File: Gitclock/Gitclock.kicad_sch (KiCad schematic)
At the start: 40 parts, among them J1 PJ-102AH, J2 Conn_01x06, J3 Conn_01x05, SW1 Omron_B3F_SPST, SW2 Omron_B3F_SPST, SW3 Omron_B3F_SPST, U1 ATmega328-PU, U2 L7805, U3 MAX7219, U4 DS1307_DIP-8, U5 WH2004A-CFH-JT#, Y1 Crystal_16MHz, Y2 Crystal_32768Hz

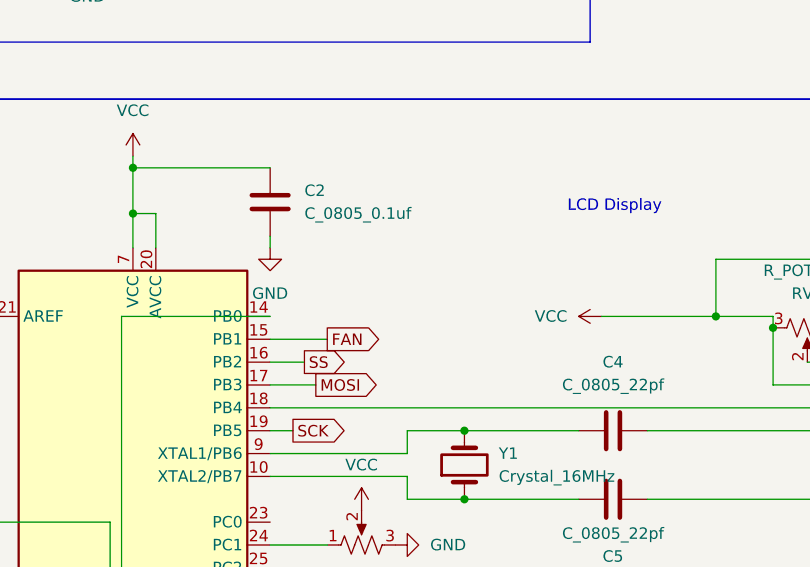
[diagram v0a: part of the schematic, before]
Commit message: gitclock
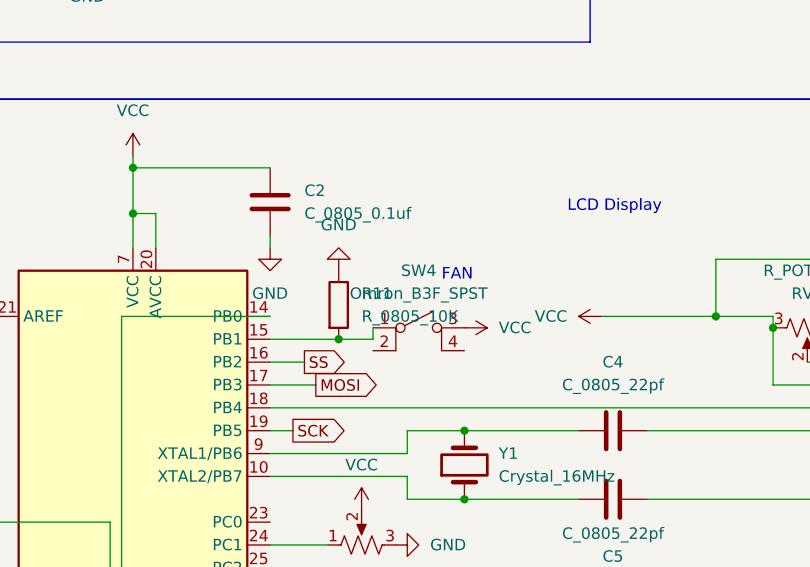
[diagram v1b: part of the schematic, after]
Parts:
- added R11: R_0805_10K, footprints:R_0805_2012Metric, symbol HPS:R_0805_10K
- added SW4: Omron_B3F_SPST, footprints:SW_SPST_Omron_B3FS-100xP, symbol HPS:Omron_B3F_SPST
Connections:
- net FAN: no longer U1.15 (PB1)
- net GND: now also R11.1
- net VCC: now also SW4.3 (B)
- new net: R11.2, SW4.1 (A), U1.15 (PB1)
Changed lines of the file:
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@@
   (junction (at 256.54 116.84) (diameter 0) (color 0 0 0 0)
+  )
+  (junction (at 203.2 99.06) (diameter 0) (color 0 0 0 0)
   )
   (no_connect (at 210.82 31.75))
@@
     (stroke (width 0) (type default) (color 0 0 0 0))
   )
+  (wire (pts (xy 207.01 99.06) (xy 207.01 97.79))
+    (stroke (width 0) (type default) (color 0 0 0 0))
+  )
   (wire (pts (xy 25.4 160.02) (xy 29.21 160.02))
     (stroke (width 0) (type default) (color 0 0 0 0))
@@
     (stroke (width 0) (type default) (color 0 0 0 0))
   )
+  (wire (pts (xy 203.2 99.06) (xy 207.01 99.06))
+    (stroke (width 0) (type default) (color 0 0 0 0))
+  )
   (wire (pts (xy 266.7 114.3) (xy 269.24 114.3))
     (stroke (width 0) (type default) (color 0 0 0 0))
@@
     (stroke (width 0) (type default) (color 0 0 0 0))
   )
-  (wire (pts (xy 195.58 99.06) (xy 201.93 99.06))
+  (wire (pts (xy 195.58 99.06) (xy 203.2 99.06))
     (stroke (width 0) (type default) (color 0 0 0 0))
   )
@@
   (text "MCU" (at 144.78 78.74 0)
     (effects (font (size 3 3)) (justify left bottom))
+  )
+  (text "FAN" (at 214.63 92.71 0)
+    (effects (font (size 1.27 1.27)) (justify left bottom))
   )
   (text "RTS\n" (at 237.49 20.32 0)
@@
     (effects (font (size 1.27 1.27)) (justify left))
     (property "Intersheet References" "${INTERSHEET_REFS}" (id 0) (at 169.4483 39.2906 0)
-      (effects (font (size 1.27 1.27)) (justify left) hide)
-    )
-  )
-  (global_label "FAN" (shape output) (at 201.93 99.06 0) (fields_autoplaced)
-    (effects (font (size 1.27 1.27)) (justify left))
-    (property "Intersheet References" "${INTERSHEET_REFS}" (id 0) (at 207.8507 98.9806 0)
       (effects (font (size 1.27 1.27)) (justify left) hide)
     )
@@
     )
     (property "Tolerance" "N/A" (id 10) (at 207.01 39.37 0)
+      (effects (font (size 1.27 1.27)) hide)
+    )
+    (pin "1")
+    (pin "2")
+  )
+  (symbol (lib_id "HPS:R_0805_10K") (at 203.2 95.25 0) (unit 1)
+    (in_bom yes) (on_board yes) (fields_autoplaced)
+    (property "Reference" "R11" (id 0) (at 205.74 93.9799 0)
+      (effects (font (size 1.27 1.27)) (justify left))
+    )
+    (property "Value" "R_0805_10K" (id 1) (at 205.74 96.5199 0)
+      (effects (font (size 1.27 1.27)) (justify left))
+    )
+    (property "Footprint" "footprints:R_0805_2012Metric" (id 2) (at 203.2 111.76 0)
+      (effects (font (size 1.27 1.27)) hide)
+    )
+    (property "Datasheet" "https://www.digikey.com/en/products/detail/yageo/RC0805FR-0710KL/727535" (id 3) (at 200.66 95.25 0)
+      (effects (font (size 1.27 1.27)) hide)
+    )
+    (property "MFG" "Yageo" (id 4) (at 203.2 106.68 0)
+      (effects (font (size 1.27 1.27)) hide)
+    )
+    (property "MPN" "RC0805FR-0710KL" (id 5) (at 203.2 109.22 0)
+      (effects (font (size 1.27 1.27)) hide)
+    )
+    (property "Digikey PN" "311-10.0KCRCT-ND" (id 6) (at 203.2 114.3 0)
+      (effects (font (size 1.27 1.27)) hide)
+    )
+    (property "Mouser PN" "N/A" (id 7) (at 203.2 116.84 0)
+      (effects (font (size 1.27 1.27)) hide)
+    )
+    (property "Power" "N/A" (id 8) (at 203.2 119.38 0)
+      (effects (font (size 1.27 1.27)) hide)
+    )
+    (property "Tolerance" "N/A" (id 9) (at 203.2 121.92 0)
       (effects (font (size 1.27 1.27)) hide)
     )
@@
     (pin "1")
     (pin "2")
+  )
+  (symbol (lib_id "HPS:Omron_B3F_SPST") (at 212.09 97.79 0) (unit 1)
+    (in_bom yes) (on_board yes) (fields_autoplaced)
+    (property "Reference" "SW4" (id 0) (at 212.09 91.44 0))
+    (property "Value" "Omron_B3F_SPST" (id 1) (at 212.09 93.98 0))
+    (property "Footprint" "footprints:SW_SPST_Omron_B3FS-100xP" (id 2) (at 212.09 109.22 0)
+      (effects (font (size 1.27 1.27)) hide)
+    )
+    (property "Datasheet" "https://omronfs.omron.com/en_US/ecb/products/pdf/en-b3fs.pdf" (id 3) (at 212.09 97.79 0)
+      (effects (font (size 1.27 1.27)) hide)
+    )
+    (property "MFG" "Omron Electronics Inc-EMC Div" (id 4) (at 212.09 104.14 0)
+      (effects (font (size 1.27 1.27)) hide)
+    )
+    (property "MPN" "B3FS-1000P" (id 5) (at 212.09 106.68 0)
+      (effects (font (size 1.27 1.27)) hide)
+    )
+    (property "Digikey PN" "SW423CT-ND" (id 6) (at 212.09 111.76 0)
+      (effects (font (size 1.27 1.27)) hide)
+    )
+    (property "Mouser PN" "N/A" (id 7) (at 212.09 114.3 0)
+      (effects (font (size 1.27 1.27)) hide)
+    )
+    (pin "1")
+    (pin "2")
+    (pin "3")
+    (pin "4")
   )
   (symbol (lib_id "HPS:Conn_01x05") (at 20.32 162.56 180) (unit 1)
@@
     )
   )
+  (symbol (lib_id "HPS:GND") (at 203.2 91.44 180) (unit 1)
+    (in_bom yes) (on_board yes) (fields_autoplaced)
+    (property "Reference" "#PWR026" (id 0) (at 203.2 85.09 0)
+      (effects (font (size 1.27 1.27)) hide)
+    )
+    (property "Value" "GND" (id 1) (at 203.2 86.36 0))
+    (property "Footprint" "" (id 2) (at 203.2 91.44 0)
+      (effects (font (size 1.27 1.27)) hide)
+    )
+    (property "Datasheet" "" (id 3) (at 203.2 91.44 0)
+      (effects (font (size 1.27 1.27)) hide)
+    )
+    (pin "1")
+  )
   (symbol (lib_id "HPS:VCC") (at 223.52 132.08 0) (unit 1)
     (in_bom yes) (on_board yes) (fields_autoplaced)
@@
     (pin "2")
   )
+  (symbol (lib_id "HPS:VCC") (at 217.17 97.79 270) (unit 1)
+    (in_bom yes) (on_board yes) (fields_autoplaced)
+    (property "Reference" "#PWR027" (id 0) (at 213.36 97.79 0)
+      (effects (font (size 1.27 1.27)) hide)
+    )
+    (property "Value" "VCC" (id 1) (at 220.98 97.7899 90)
+      (effects (font (size 1.27 1.27)) (justify left))
+    )
+    (property "Footprint" "" (id 2) (at 217.17 97.79 0)
+      (effects (font (size 1.27 1.27)) hide)
+    )
+    (property "Datasheet" "" (id 3) (at 217.17 97.79 0)
+      (effects (font (size 1.27 1.27)) hide)
+    )
+    (pin "1")
+  )
   (symbol (lib_id "HPS:GND") (at 165.1 146.05 0) (unit 1)
     (in_bom yes) (on_board yes) (fields_autoplaced)
@@
       (reference "#PWR025") (unit 1) (value "VCC") (footprint "")
     )
+    (path "/b2f7aa7c-1b8a-4b2a-b447-22be93212478"
+      (reference "#PWR026") (unit 1) (value "GND") (footprint "")
+    )
+    (path "/fcda8e25-b4ca-4300-bca3-4f296e33f7cc"
+      (reference "#PWR027") (unit 1) (value "VCC") (footprint "")
+    )
     (path "/b8ab70f2-d09f-4473-ad37-89ea941dca60"
       (reference "BZ1") (unit 1) (value "Buzzer") (footprint "footprints:Buzzer_TDK_PS1240P02BT_D12.2mm_H6.5mm")
@@
       (reference "R10") (unit 1) (value "R_0805_1K") (footprint "footprints:R_0805_2012Metric")
     )
+    (path "/17ccefeb-a492-427b-8efd-13f0e4786ae3"
+      (reference "R11") (unit 1) (value "R_0805_10K") (footprint "footprints:R_0805_2012Metric")
+    )
     (path "/99c06508-6a16-489f-a186-ced706cf79b5"
       (reference "RV1") (unit 1) (value "R_POT_10K") (footprint "footprints:Potentiometer_Bourns_3386P_Vertical")
@@
       (reference "SW3") (unit 1) (value "Omron_B3F_SPST") (footprint "footprints:SW_SPST_Omron_B3FS-100xP")
     )
+    (path "/5f30d32f-818b-4e3a-9a53-1ff51ebb71a9"
+      (reference "SW4") (unit 1) (value "Omron_B3F_SPST") (footprint "footprints:SW_SPST_Omron_B3FS-100xP")
+    )
     (path "/69182d8d-4416-465a-9377-142ba3779f64"

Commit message: gitclock6302022
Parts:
- removed R10, R7: R_0805_1K, footprints:R_0805_2012Metric, symbol HPS:R_0805_1K
- removed RV2, RV3: R_POT_10K, footprints:Potentiometer_Bourns_3386P_Vertical, symbol HPS:R_POT_10K
- removed U5: WH2004A-CFH-JT#, footprints:WH2004A-CFH-JT#, symbol HPS:WH2004A-CFH-JT#
- added BT1: Battery_Cell, footprints:BatteryHolder_Keystone_106_1x20mm, symbol HPS:Battery_Cell
- added DS2: TC1602A-01T, footprints:TC1602A-01T, symbol HPS:TC1602A-01T
- added SW5: RotaryEncoder_Switch, footprints:RotaryEncoder_TT_EN11-Switch_Vertical_H20mm_CircularMountingHoles, symbol HPS:RotaryEncoder_Switch
- added U5: ULN2003A, footprints:DIP-16_W7.62mm, symbol HPS:ULN2003A
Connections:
- net +BATT: now also BT1.1 (+)
- net FAN: now also BZ1.2 (+), R11.2, SW4.1 (A), U1.15 (PB1); no longer J3.4 (Pin_4)
- net GND: now also BT1.2 (-), DS2.1 (VSS), DS2.16 (LED(-)), DS2.5 (R/W), SW5.C, U5.8 (GND)
- net MOSI: now also DS2.6 (E)
- net SCL: now also SW5.A
- net VCC: now also DS2.15 (LED(+)), DS2.2 (VDD), SW5.S1, U5.9 (COM); no longer SW4.3 (B)
- net SNOOZE: now reaches R6.1, SW2.3 (B), U1.14 (PB0)
- net BUZZER: now reaches U1.12 (PD6)
- net D7: now reaches U1.11 (PD5)
- net D7: now also DS2.14 (D7)
- net MENU: now reaches R5.1, SW3.3 (B), U1.13 (PD7)
- net RS: now reaches U1.18 (PB4)
- net RS: now also DS2.4 (RS)
- net MENU SCROLL: now reaches U1.24 (PC1)
- net MENU SCROLL: now also SW5.B
- net D4: now reaches U1.4 (PD2)
- net D4: now also DS2.11 (D4)
- net D5: now reaches U1.5 (PD3)
- net D5: now also DS2.12 (D5)
- net D6: now reaches U1.6 (PD4)
- net D6: now also DS2.13 (D6)
- new net: SW4.3 (B), U5.1 (I1)
- new net: J3.4 (Pin_4), U5.16 (O1)
- no-connect marks 13 -> 25
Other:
- note added: "BUZZER"
- note added: "MENU"
- note added: "MENU SCROLL"
- note removed: "SETTINGS"
- moved on the sheet: BZ1, C1, C2, C3, C4, C5, C6, C7, D1, DS1, H3, H4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
